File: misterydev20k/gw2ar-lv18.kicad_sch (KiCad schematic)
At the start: 53 parts, among them J3 JTAG, U11 TLV62569DBV, U5 GW2AR-LV18-QN88, U6 W25Q128JVS, U8 ME6211C33M5, U9 ME6211C33M5, Y2 27MHz

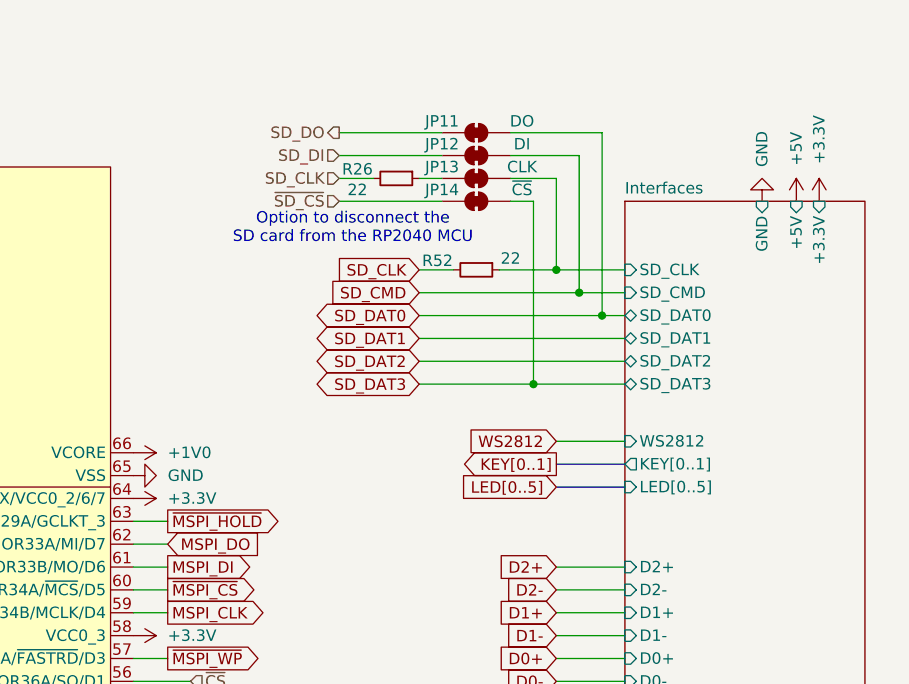
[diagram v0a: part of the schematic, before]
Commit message: Update missing files
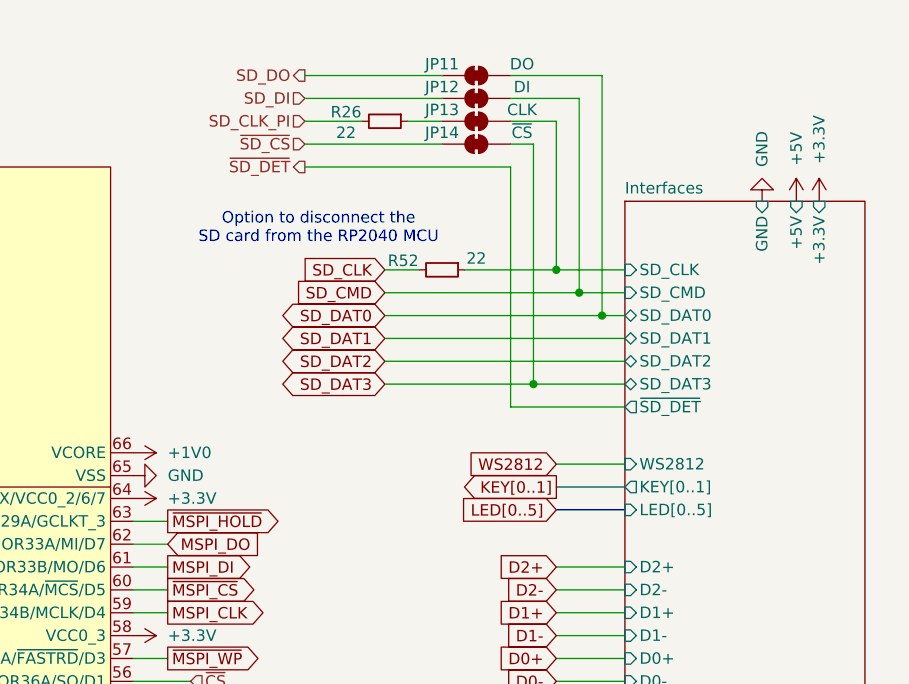
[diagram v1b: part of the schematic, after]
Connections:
- net SD_CLK: no longer R26.2
- new net SD_CLK_PI: R26.2
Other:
- sheet Interfaces ports: added ~{SD_DET}; removed none
- moved on the sheet: JP11, JP12, JP13, JP14, R26, R52
